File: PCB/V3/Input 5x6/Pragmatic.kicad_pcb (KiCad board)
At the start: 2 copper layers, 114.3 x 108 mm, 70 parts, among them J1 Hand-Soldering, SW1 SW_Push, SW10 SW_Push, SW11 SW_Push, SW12 SW_Push, SW13 SW_Push, SW14 SW_Push, SW15 SW_Push, SW16 SW_Push, SW17 SW_Push, SW18 SW_Push, SW19 SW_Push, SW2 SW_Push, SW20 SW_Push, SW21 SW_Push, SW22 SW_Push, SW23 SW_Push, SW24 SW_Push, SW25 SW_Push, SW26 SW_Push, SW27 SW_Push, SW28 SW_Push, SW29 SW_Push, SW3 SW_Push, SW30 SW_Push, SW4 SW_Push, SW5 SW_Push, SW6 SW_Push, SW7 SW_Push, SW8 SW_Push, SW9 SW_Push

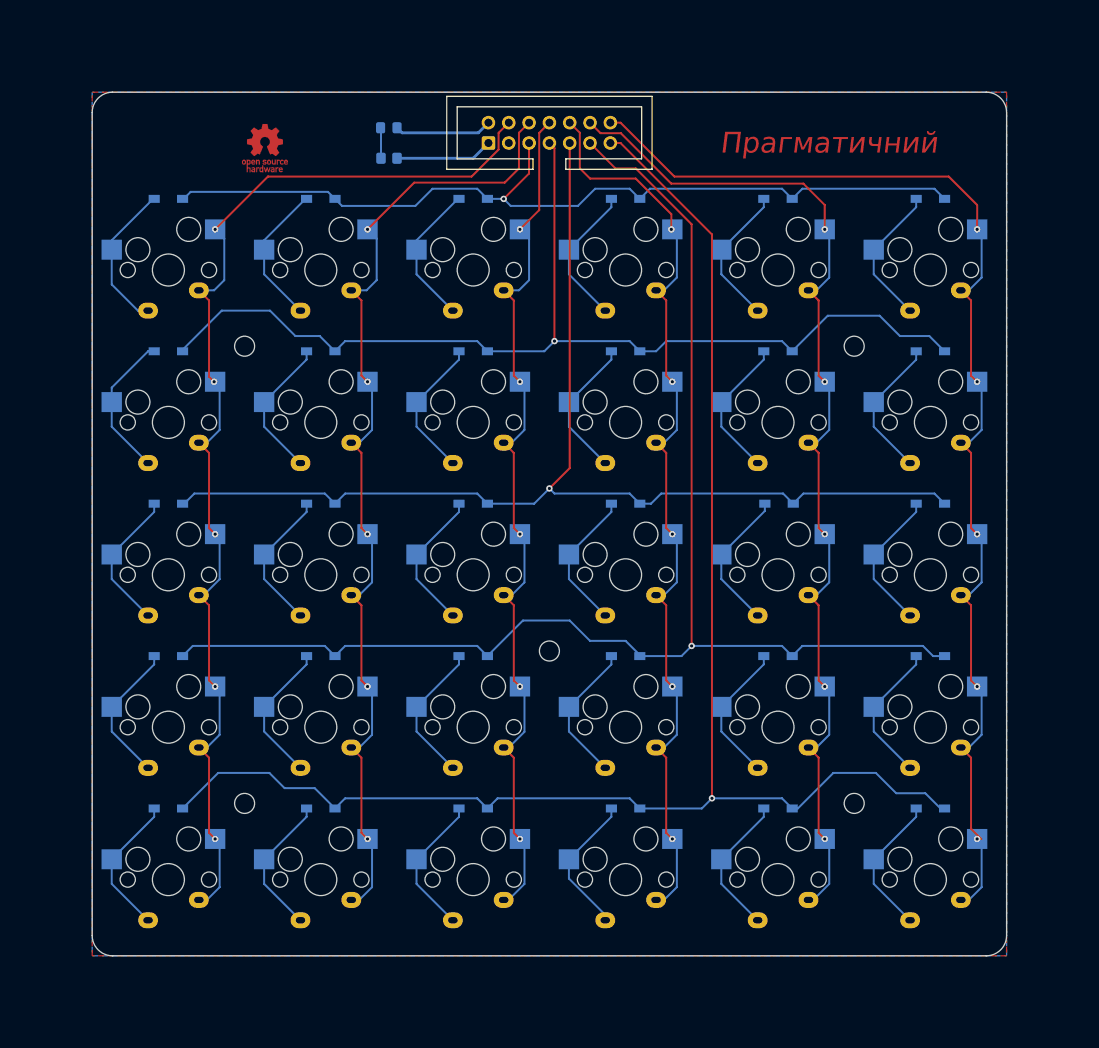
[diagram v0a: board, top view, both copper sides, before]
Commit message: 60 plate
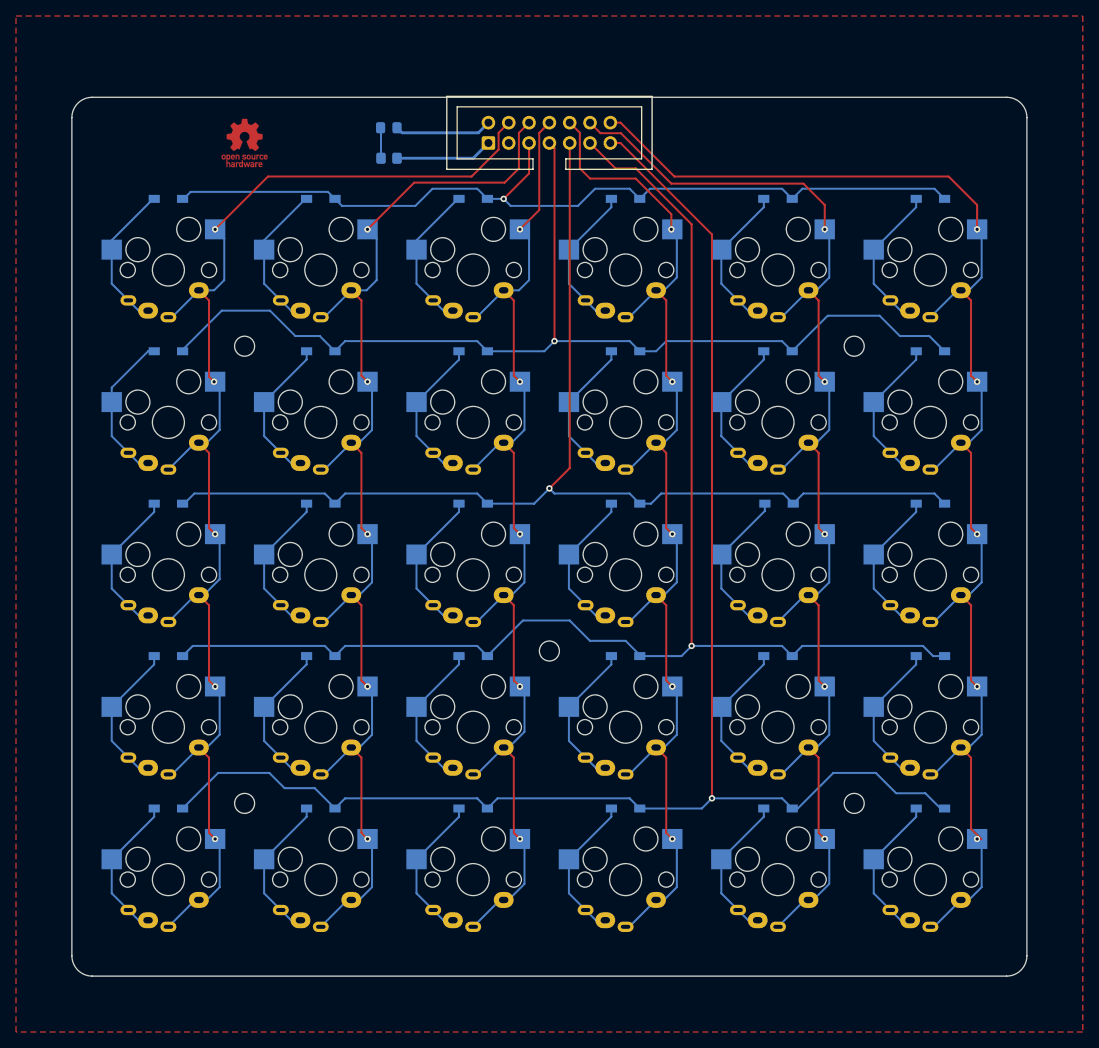
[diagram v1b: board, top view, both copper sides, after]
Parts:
- SW1, SW10, SW11, SW12, SW13, SW14, SW15, SW16, SW17, SW18, SW19, SW2, SW20, SW21, SW22, SW23, SW24, SW25, SW26, SW27, SW28, SW29, SW3, SW30, SW4, SW5, SW6, SW7, SW8, SW9: footprint Keyboard_JSA:CherryMX_Hotswap -> Keyboard_JSA:MX_Hotswap_MX_Choc_Solder
- moved LOGO1 2.62 mm to (66.7, 41.3)
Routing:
- net Col5: track 133.1 -> 159.1 mm
- net Col4: track 118.6 -> 144.6 mm
- net Col3: track 112.1 -> 138.1 mm
- net Col6: track 150.5 -> 176.5 mm
- net Col2: track 126.0 -> 152.0 mm
- net Col1: track 140.9 -> 166.9 mm
- net Net-(D23-Pad2): track 18.1 -> 18.7 mm
- net Net-(D16-Pad2): track 18.1 -> 18.7 mm
- net Net-(D7-Pad2): track 18.5 -> 19.2 mm
- net Net-(D6-Pad2): track 18.1 -> 18.7 mm
- net Net-(D30-Pad2): track 18.1 -> 18.7 mm
- net Net-(D29-Pad2): track 18.1 -> 18.7 mm
- net Net-(D28-Pad2): track 18.1 -> 18.7 mm
- net Net-(D25-Pad2): track 18.1 -> 18.7 mm
- net Net-(D24-Pad2): track 18.1 -> 18.7 mm
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- removed copper zone on B.Cu, net (none)
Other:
- board size 114.3 x 108 mm -> 119.4 x 109.9 mm
- board text added: "V3.1"
- board text removed: "V3 Hotswap"
